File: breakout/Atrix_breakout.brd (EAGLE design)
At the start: 13.3 x 18.9 mm, 5 parts

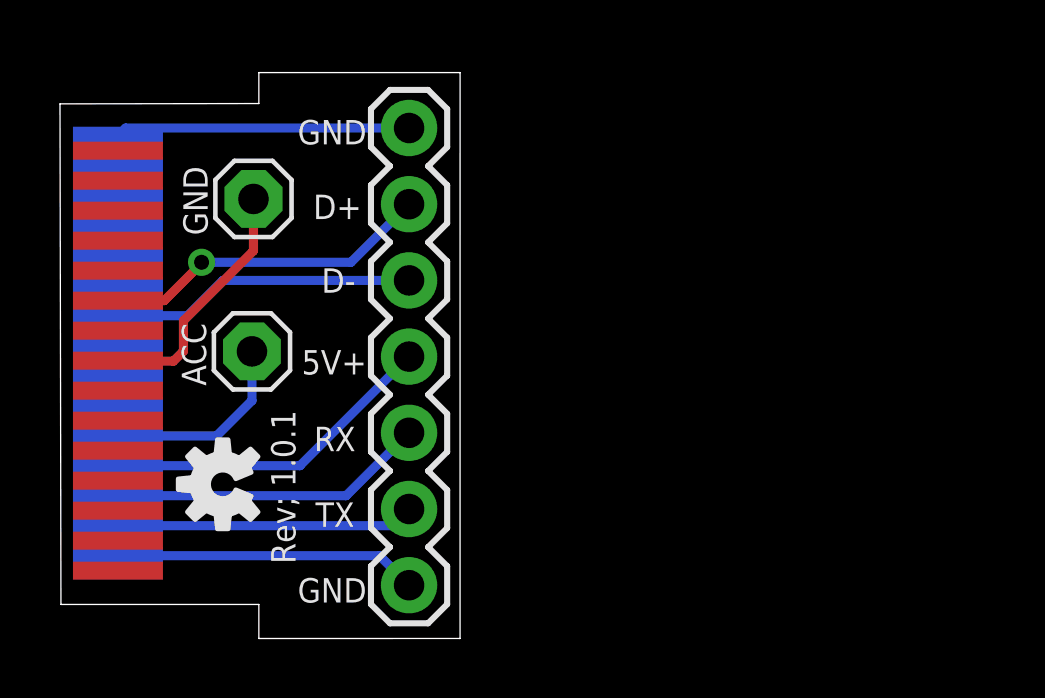
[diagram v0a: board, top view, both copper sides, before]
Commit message: Rev v1.0.2r2
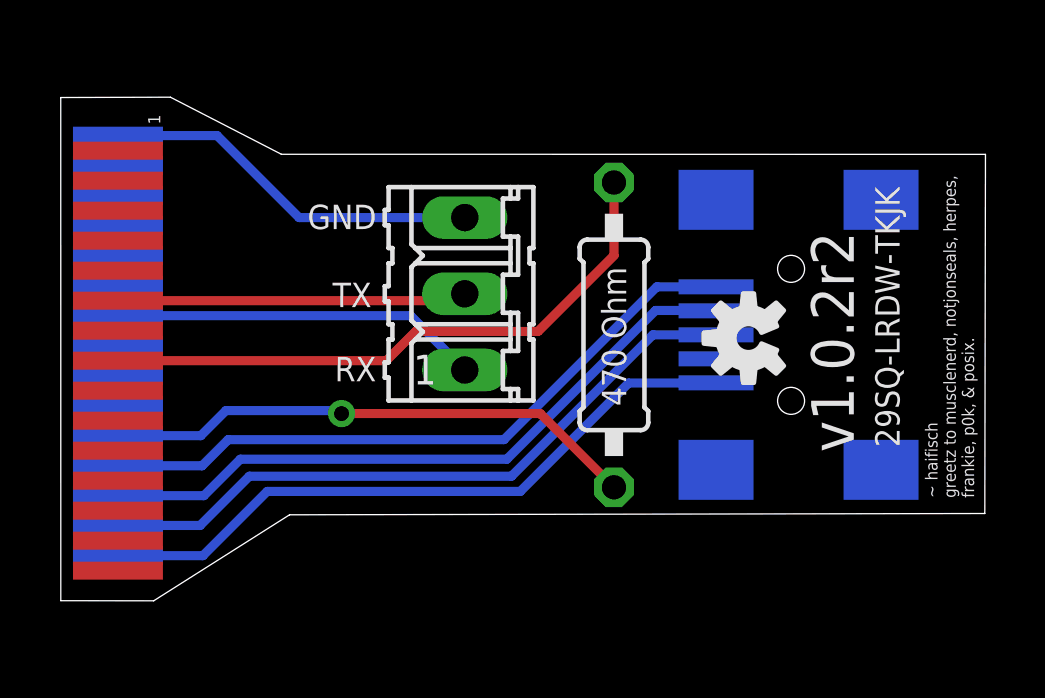
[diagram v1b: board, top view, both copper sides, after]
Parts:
- removed ACC, GND: (no value), adafruit:1X01
- added R1: (no value), eagle-ltspice:0207/10
- added U$3: USB-MINIB-5PIN, SparkFun-Connectors:USB-MINIB
- JP1: device SparkFun-Connectors:1X07 -> con-amp-quick:03P
- moved U$2 18.2 mm to (21.3, 12.8)
- moved JP1 9.89 mm to (11.9, 14.3)
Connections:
- net 5V+: now also U$3.VBUS; no longer JP1.4
- net ACC: now also R1.2; no longer ACC.1
- net ACC_GROUND: now also R1.1; no longer GND.1
- net D+: now also U$3.D+; no longer JP1.2
- net D-: now also U$3.D-; no longer JP1.3
- net GND: now also JP1.3; no longer JP1.7
- net RX: now also JP1.1; no longer JP1.5
- net TX: now also JP1.2; no longer JP1.6
- net USB_GND: now also U$3.GND; no longer JP1.1
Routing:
- net D+: track 9.93 -> 22.6 mm
- net USB_GND: track 10.1 -> 22.3 mm
- net ACC_GROUND: track 8.37 -> 20.4 mm
- net D-: track 10.6 -> 22.5 mm
- net ACC: track 6.60 -> 17.9 mm, vias 0 -> 1
- net 5V+: track 11.2 -> 22.4 mm
- net GND: track 9.81 -> 12.7 mm
- net RX: track 10.2 -> 12.3 mm
- net TX: track 11.1 -> 11.7 mm, vias 1 -> 0
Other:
- board size 13.3 x 18.9 mm -> 30.8 x 16.8 mm
- board text added: "1"
- board text added: "29SQ-LRDW-TKJK"
- board text added: "470 Ohm"
- board text added: "v1.0.2r2"
- board text added: "~ haifisch greetz to musclenerd, notjonseals, herpes, frankie, p0k, & posix."
- board text removed: "5V+"
- board text removed: "D+"
- board text removed: "D-"
- board text removed: "Rev; 1.0.1"
